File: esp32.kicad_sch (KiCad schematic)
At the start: 36 parts, among them SW2 BOOT, U6 ESP32-S3R8, U7 W25Q128JVSIQ, Y1 40MHz

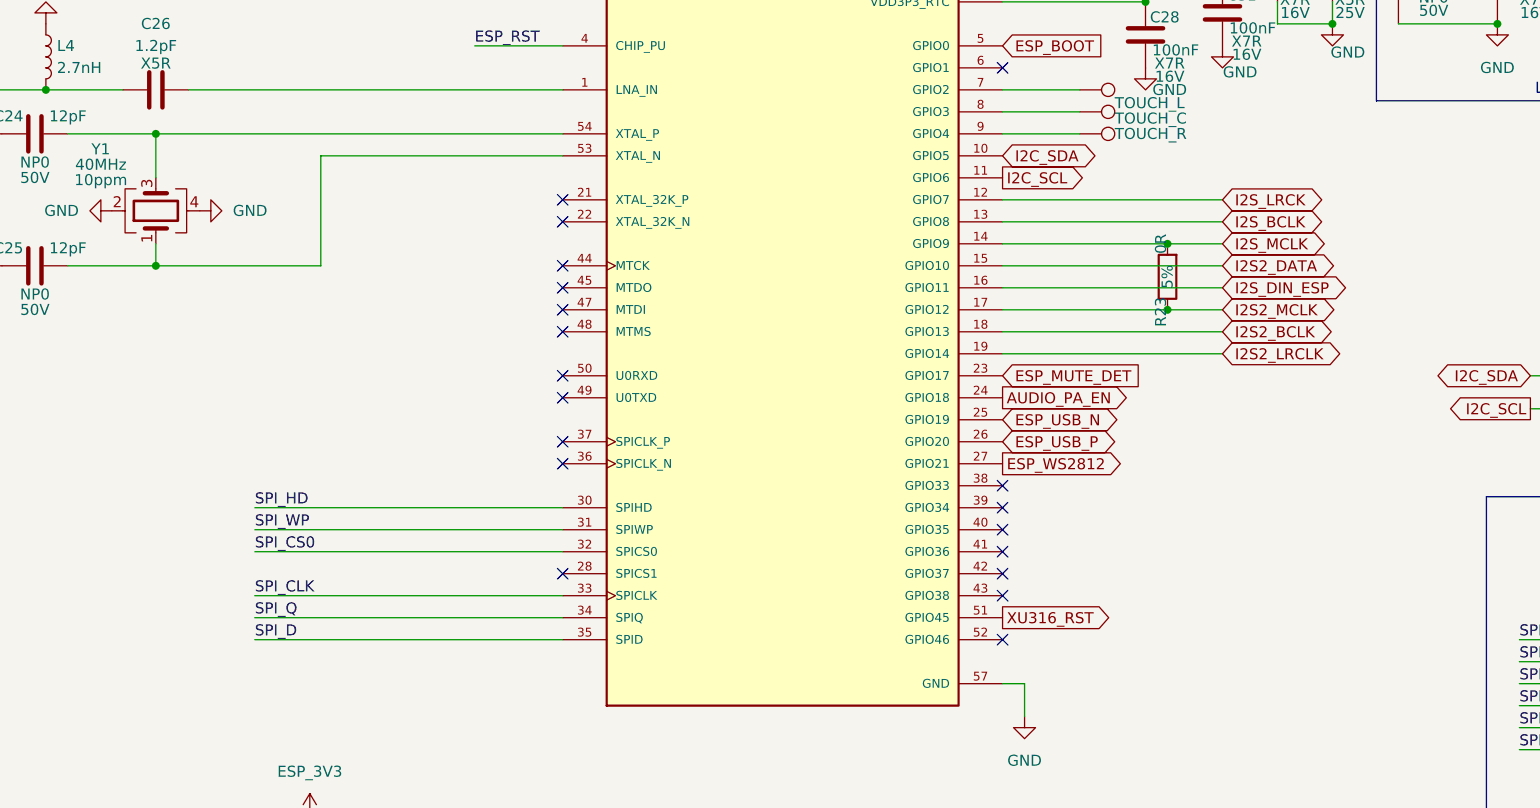
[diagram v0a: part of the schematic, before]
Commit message: routing
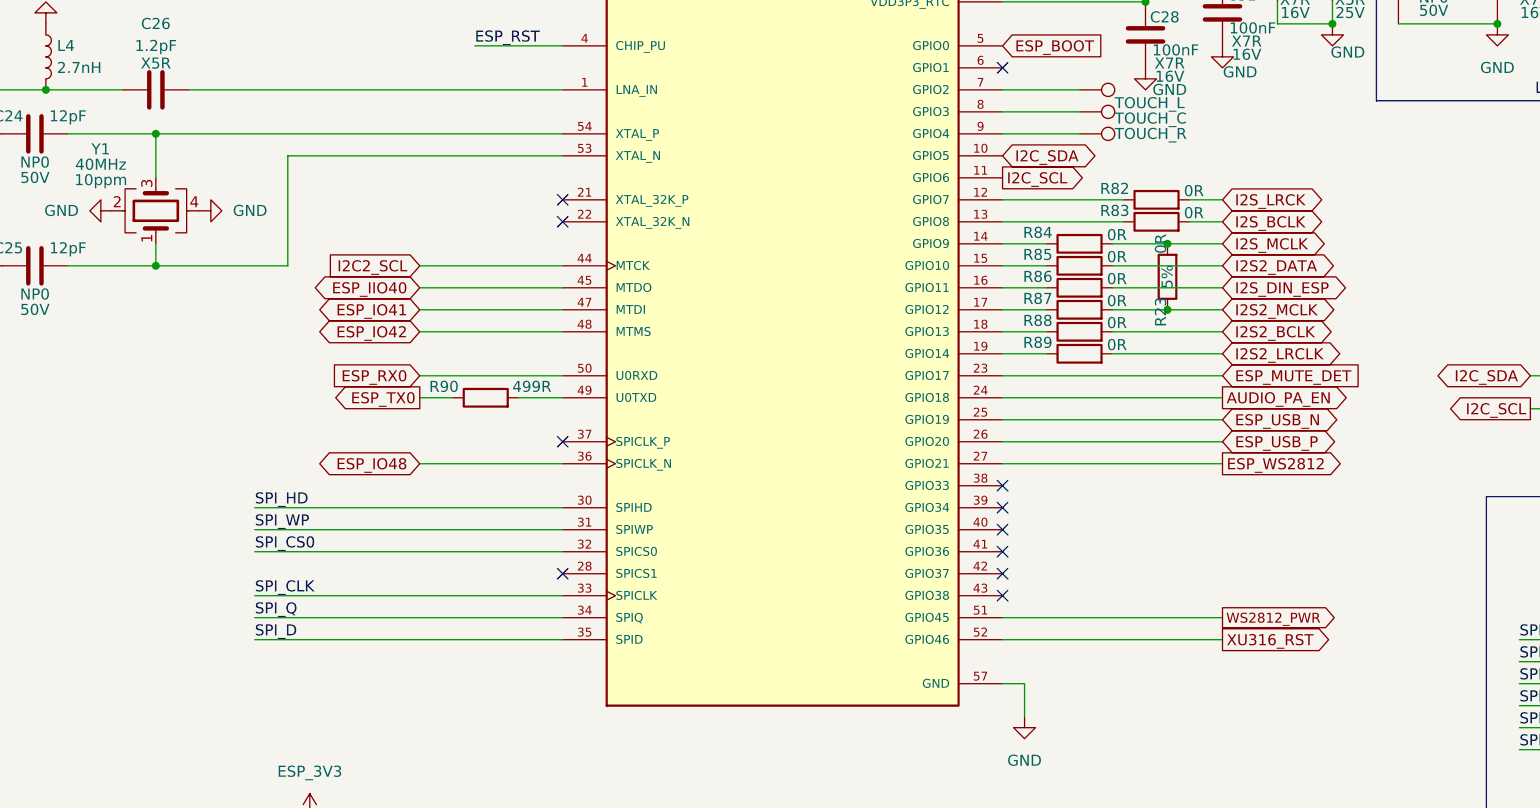
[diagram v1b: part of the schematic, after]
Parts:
- added R82, R83, R84, R85, R86, R87, R88, R89: 0R, Resistor_SMD:R_0402_1005Metric, symbol Device:R
- added R90: 499R, Resistor_SMD:R_0402_1005Metric, symbol Device:R
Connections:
- net I2S2_BCLK: now also R88.2; no longer U6.18 (GPIO13)
- net I2S2_DATA: now also R85.2; no longer U6.15 (GPIO10)
- net I2S2_LRCLK: now also R89.2; no longer U6.19 (GPIO14)
- net I2S2_MCLK: now also R87.2; no longer U6.17 (GPIO12)
- net I2S_BCLK: now also R83.2; no longer U6.13 (GPIO8)
- net I2S_DIN_ESP: now also R86.2; no longer U6.16 (GPIO11)
- net I2S_LRCK: now also R82.2; no longer U6.12 (GPIO7)
- net I2S_MCLK: now also R84.2; no longer U6.14 (GPIO9)
- net XU316_RST: now also U6.52 (GPIO46); no longer U6.51 (GPIO45)
- net ESP_IO48: now reaches U6.36 (SPICLK_N)
- net I2C2_SCL: now reaches U6.44 (MTCK)
- net ESP_IIO40: now reaches U6.45 (MTDO)
- net ESP_IO41: now reaches U6.47 (MTDI)
- net ESP_IO42: now reaches U6.48 (MTMS)
- net at U6.49 (U0TXD): now also R90.2
- net ESP_RX0: now reaches U6.50 (U0RXD)
- new net: R83.1, U6.13 (GPIO8)
- new net: R89.1, U6.19 (GPIO14)
- new net: R82.1, U6.12 (GPIO7)
- new net: R84.1, U6.14 (GPIO9)
- new net: R85.1, U6.15 (GPIO10)
- new net: R86.1, U6.16 (GPIO11)
- new net: R87.1, U6.17 (GPIO12)
- new net: R88.1, U6.18 (GPIO13)
- new net ESP_TX0: R90.1
- new net WS2812_PWR: U6.51 (GPIO45)
- no-connect marks 19 -> 11

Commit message: routing
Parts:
- Y1: footprint Crystal:Crystal_SMD_3225-4Pin_3.2x2.5mm -> Crystal:Crystal_SMD_2016-4Pin_2.0x1.6mm; LCSC Part # C9010 -> (none); Manufacturer YXC Crystal Oscillators -> Murata; Manufacturer Part X322540MPB4SI -> XRCGB40M000F1S2SR0
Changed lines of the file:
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@@
 			)
 		)
-		(property "Footprint" "Crystal:Crystal_SMD_3225-4Pin_3.2x2.5mm"
+		(property "Footprint" "Crystal:Crystal_SMD_2016-4Pin_2.0x1.6mm"
 			(at 64.77 85.09 0)
 			(effects
@@
 			)
 		)
-		(property "Datasheet" "~"
+		(property "Datasheet" ""
 			(at 64.77 85.09 0)
 			(effects
@@
 			)
 		)
-		(property "Description" "±10ppm, 18pF, 50Ω, ABM8G-40.000MHZ-B2-T"
+		(property "Description" "40 MHz ±10ppm Crystal 9pF 50 Ohms 4-SMD, No Lead"
 			(at 64.77 85.09 0)
 			(effects
@@
 			)
 		)
-		(property "LCSC Part #" "C9010"
+		(property "LCSC Part #" ""
 			(at 64.77 85.09 90)
 			(effects
@@
 			)
 		)
-		(property "Manufacturer" "YXC Crystal Oscillators"
+		(property "Manufacturer" "Murata"
 			(at 64.77 85.09 90)
 			(effects
@@
 			)
 		)
-		(property "Manufacturer Part" "X322540MPB4SI"
+		(property "Manufacturer Part" "XRCGB40M000F1S2SR0"
 			(at 64.77 85.09 90)
 			(effects
